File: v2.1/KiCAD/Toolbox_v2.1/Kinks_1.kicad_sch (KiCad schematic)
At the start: 22 parts, among them J26 Kinks_OUT_MAX, J27 Kinks_IN_A, J28 Kinks_IN_B, J29 Kinks_OUT_MIN, U6 TL074, U7 TL074

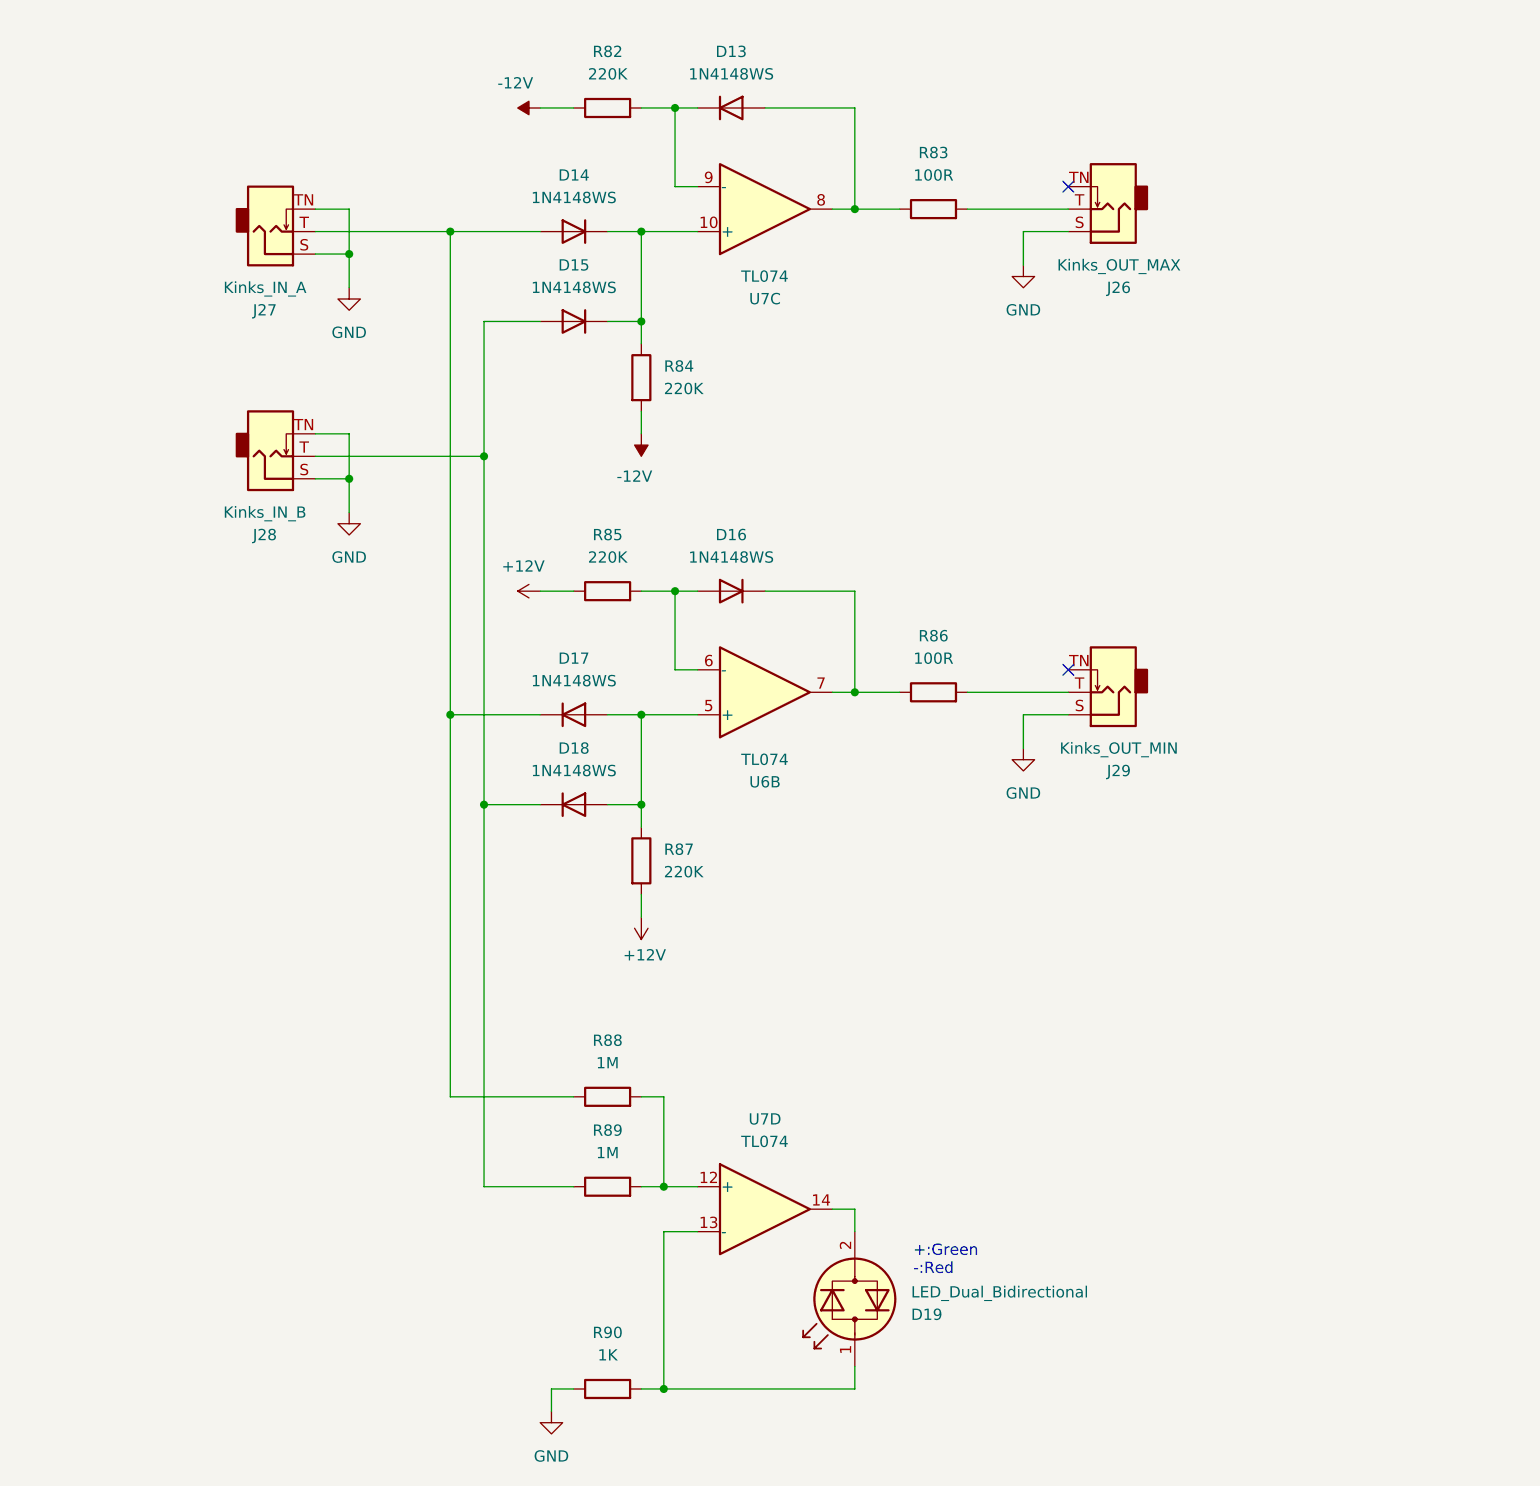
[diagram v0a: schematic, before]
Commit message: v2.1 Update
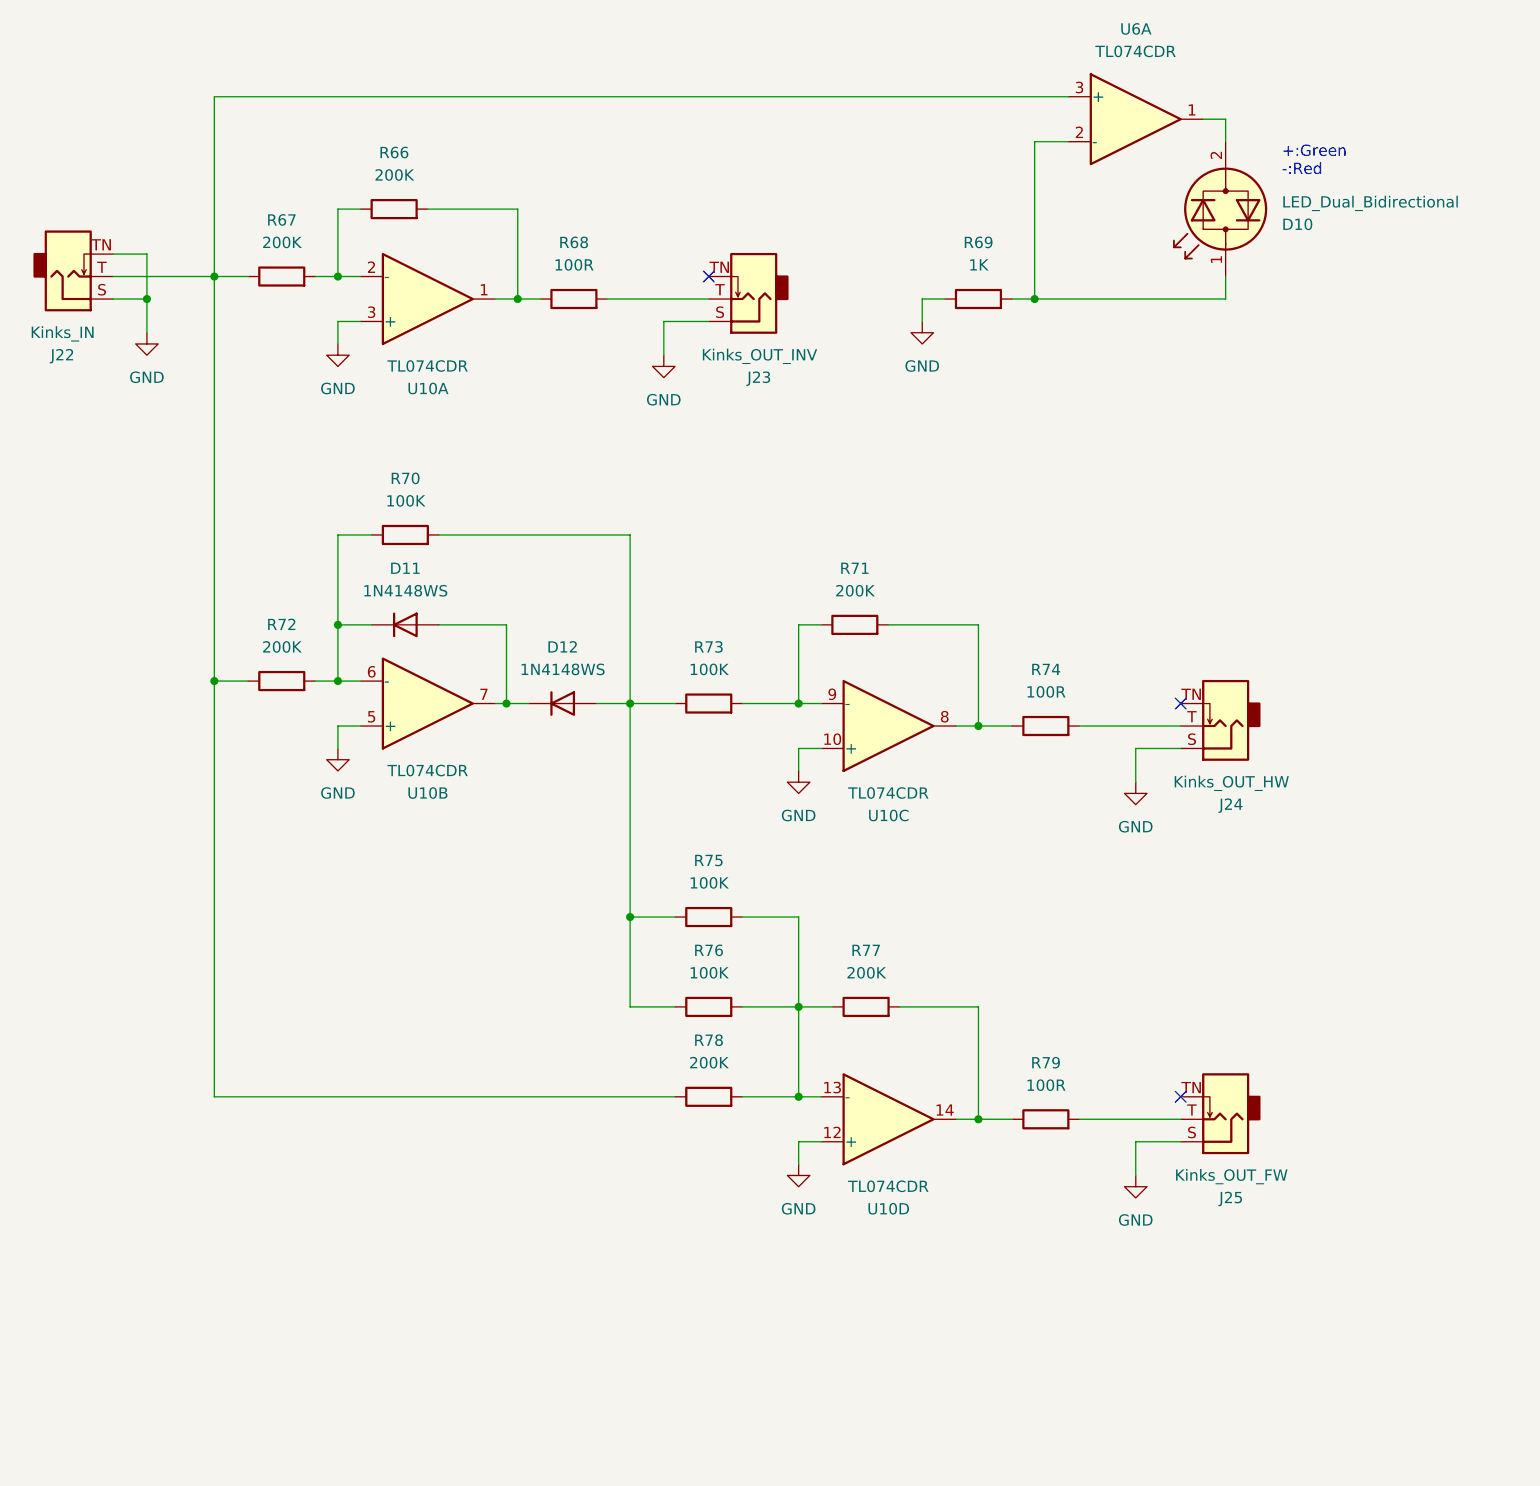
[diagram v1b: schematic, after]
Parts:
- removed D13, D14, D15, D16, D17, D18: 1N4148WS, Diode_SMD:D_SOD-323, symbol Diode:1N4148WS
- removed D19: LED_Dual_Bidirectional, LED_THT:LED_D3.0mm, symbol Device:LED_Dual_Bidirectional
- removed J26: Kinks_OUT_MAX, kat_eurorack:AudioJack_PJ301M-12, symbol Connector_Audio:AudioJack2_SwitchT
- removed J27: Kinks_IN_A, kat_eurorack:AudioJack_PJ301M-12, symbol Connector_Audio:AudioJack2_SwitchT
- removed J28: Kinks_IN_B, kat_eurorack:AudioJack_PJ301M-12, symbol Connector_Audio:AudioJack2_SwitchT
- removed J29: Kinks_OUT_MIN, kat_eurorack:AudioJack_PJ301M-12, symbol Connector_Audio:AudioJack2_SwitchT
- removed R82, R84, R85, R87: 220K, Resistor_SMD:R_0402_1005Metric, symbol Device:R
- removed R83, R86: 100R, Resistor_SMD:R_0402_1005Metric, symbol Device:R
- removed R88, R89: 1M, Resistor_SMD:R_0402_1005Metric, symbol Device:R
- removed R90: 1K, Resistor_SMD:R_0402_1005Metric, symbol Device:R
- removed U6, U7: TL074, Package_SO:TSSOP-14_4.4x5mm_P0.65mm, symbol Amplifier_Operational:TL074
- added D10: LED_Dual_Bidirectional, LED_THT:LED_D3.0mm, symbol Device:LED_Dual_Bidirectional
- added D11, D12: 1N4148WS, Diode_SMD:D_SOD-323, symbol Diode:1N4148WS
- added J22: Kinks_IN, kat_eurorack:AudioJack_PJ301M-12, symbol Connector_Audio:AudioJack2_SwitchT
- added J23: Kinks_OUT_INV, kat_eurorack:AudioJack_PJ301M-12, symbol Connector_Audio:AudioJack2_SwitchT
- added J24: Kinks_OUT_HW, kat_eurorack:AudioJack_PJ301M-12, symbol Connector_Audio:AudioJack2_SwitchT
- added J25: Kinks_OUT_FW, kat_eurorack:AudioJack_PJ301M-12, symbol Connector_Audio:AudioJack2_SwitchT
- added R66, R67, R71, R72, R77, R78: 200K, Resistor_SMD:R_0402_1005Metric, symbol Device:R
- added R68, R74, R79: 100R, Resistor_SMD:R_0402_1005Metric, symbol Device:R
- added R69: 1K, Resistor_SMD:R_0402_1005Metric, symbol Device:R
- added R70, R73, R75, R76: 100K, Resistor_SMD:R_0402_1005Metric, symbol Device:R
- added U10, U6: TL074CDR, Package_SO:SOIC-14_3.9x8.7mm_P1.27mm, symbol Amplifier_Operational:TL074
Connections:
- net GND: now also J22.S, J22.TN, J23.S, J24.S, J25.S, R69.1, U10.10 (+), U10.12 (+), U10.3 (+), U10.5 (+)
- new net: D11.1 (K), R70.1, R72.2, U10.6 (-)
- new net: D11.2 (A), D12.1 (K), U10.7
- new net: R75.2, R76.2, R77.1, R78.2, U10.13 (-)
- new net: R77.2, R79.1, U10.14
- new net: J25.T, R79.2
- new net: J22.T, R67.1, R72.1, R78.1, U6.3 (+)
- new net: D12.2 (A), R70.2, R73.1, R75.1, R76.1
- new net: R71.2, R74.1, U10.8
- new net: R71.1, R73.2, U10.9 (-)
- new net: R66.2, R68.1, U10.1
- new net: R66.1, R67.2, U10.2 (-)
- new net: J24.T, R74.2
- new net: D10.1 (KA), R69.2, U6.2 (-)
- new net: D10.2 (AK), U6.1
- new net: J23.T, R68.2
- no-connect marks 2 -> 3
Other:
- title: Analog AND/OR -> HW/FW rectifiers
